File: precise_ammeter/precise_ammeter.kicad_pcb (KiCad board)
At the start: 2 copper layers, 94.9 x 63.9 mm, 105 parts, among them J1 Conn_01x01_Socket, J2 Conn_01x01_Socket, J3 USB4110GFA, J4 Conn_ARM_JTAG_SWD_10, U1 INA121U, U11 STM32G431C6Tx, U12 USBLC6-2P6, U2 TLV9301xDBV, U3 TLV9301xDBV, U4 INA137UA, U5 OPA376xxD, U6 OPA376xxD, U7 TPS7A2433DBVR, U9 LMC7660, Y1 Crystal

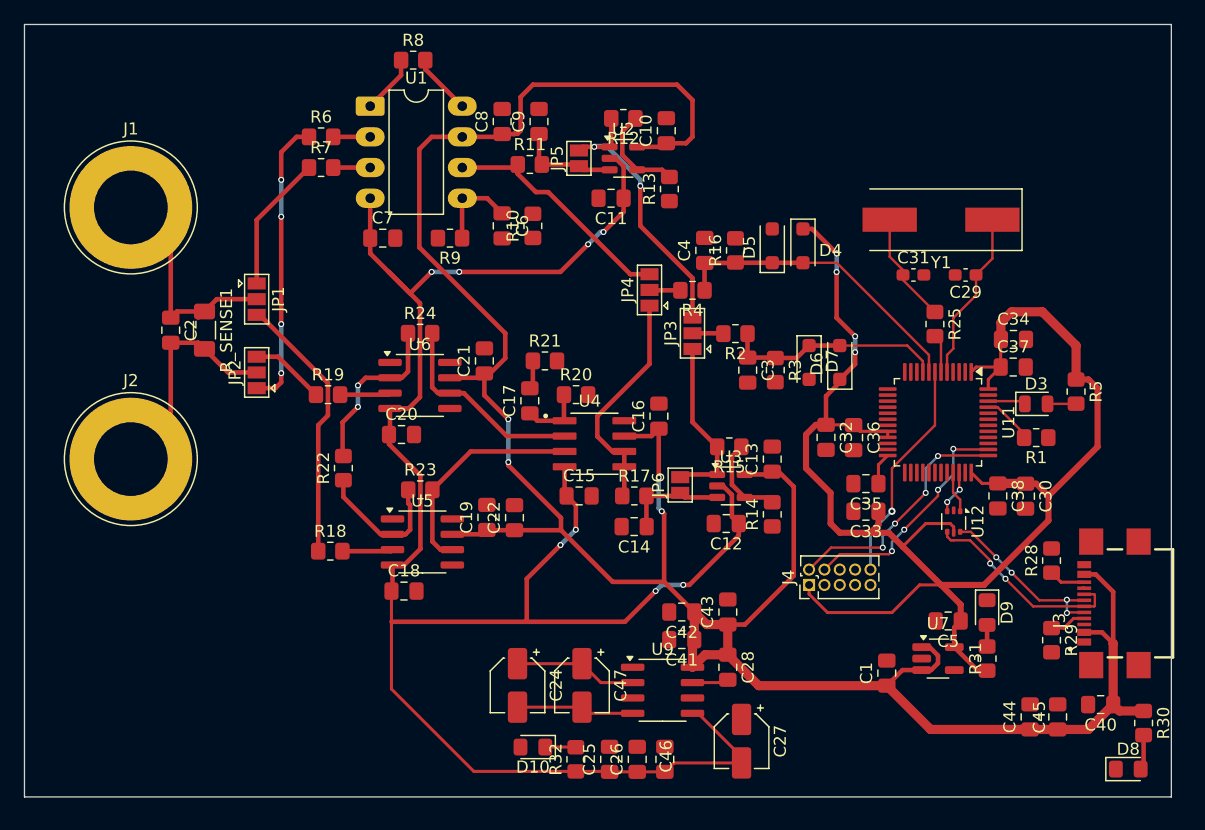
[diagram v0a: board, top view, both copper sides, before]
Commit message: dodano skonczone PCB
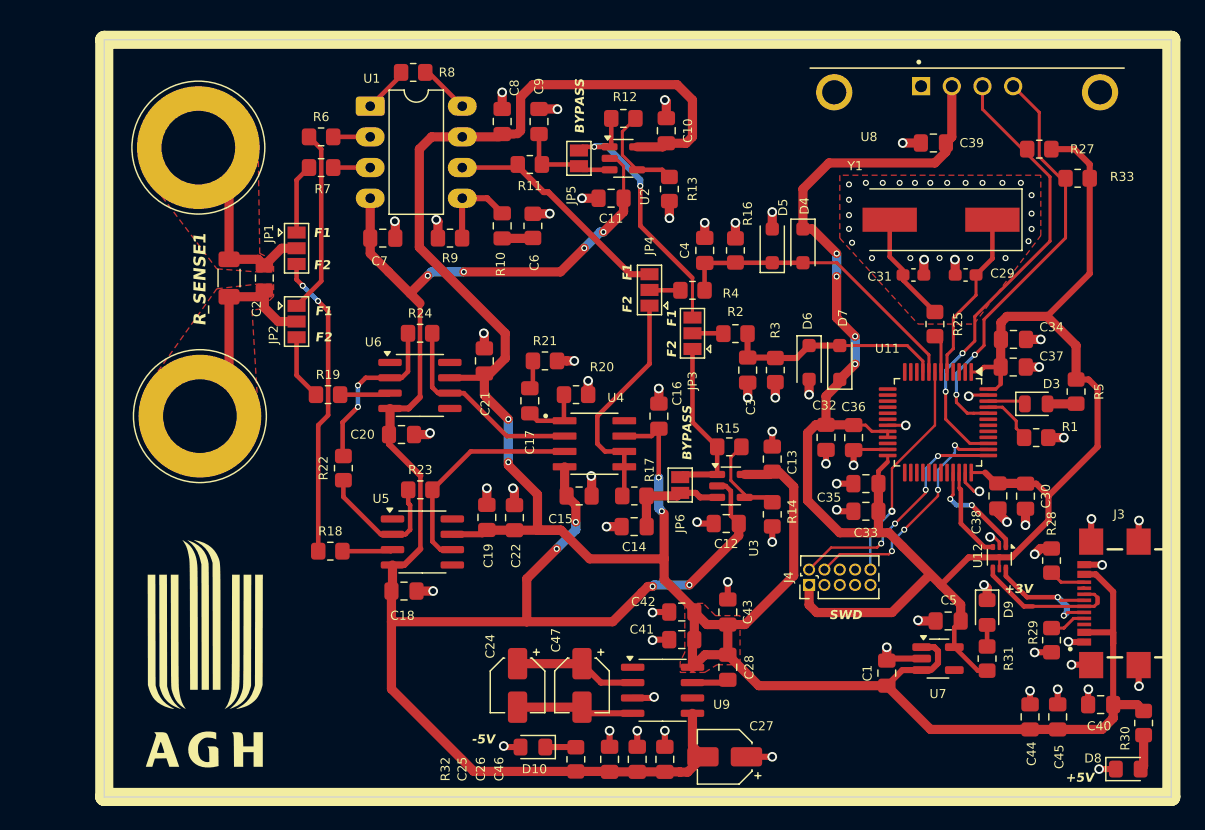
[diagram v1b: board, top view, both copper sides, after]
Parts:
- added C39: 1u, Capacitor_SMD:C_0805_2012Metric_Pad1.18x1.45mm_HandSolder, F.Cu at (213.7, 91.2)
- added G***: LOGO, LOGO, F.Cu at (153.4, 133.5)
- added R27: 4.7k, Resistor_SMD:R_0805_2012Metric_Pad1.20x1.40mm_HandSolder, F.Cu at (222.5, 91.7)
- added R33: 4.7k, Resistor_SMD:R_0805_2012Metric_Pad1.20x1.40mm_HandSolder, F.Cu at (225.7, 94.1)
- added U8: DM-OLED096-636, DM-OLED096-636:MODULE_DM-OLED096-636, F.Cu at (216.5, 98.0)
- moved C2 8.87 mm to (158.4, 102.4)
- moved J1 7.47 mm to (152.9, 91.6)
- moved J2 6.73 mm to (153.0, 113.8)
- moved JP1 5.35 mm to (161.0, 99.9)
- moved JP2 5.35 mm to (161.0, 106.0), turned to -90 degrees
- moved U12 4.80 mm to (219.2, 125.5)
- moved R_SENSE1 4.77 mm to (155.4, 102.4)
- moved C27 1.90 mm to (196.5, 142.0), turned to 180 degrees
- moved R8 1.02 mm to (170.7, 85.3)
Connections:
- U11 pad 39: unconnected-(U11-PA15-Pad39) -> /MCU/SCL
- U11 pad 44: unconnected-(U11-PB7-Pad44) -> /MCU/SDA
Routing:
- net GND: track 0.00 -> 101.1 mm, vias 0 -> 91
- net /MCU/SCL: track 0.00 -> 38.0 mm, vias 0 -> 2
- net +3V3: track 132.2 -> 170.0 mm
- net /MCU/SDA: track 0.00 -> 34.9 mm, vias 0 -> 2
- net /Curr_measurement/Frontend_1/Frontend_1_IN-: track 24.1 -> 15.2 mm, vias 4 -> 0
- net /Curr_measurement/Frontend_1/Frontend_1_IN+: track 11.4 -> 5.81 mm
- net Net-(U11-PA11): track 3.45 -> 9.00 mm, vias 0 -> 2
- net /MCU/USB_D_P: track 17.0 -> 12.2 mm, vias 2 -> 0
- net -5VA: track 165.0 -> 160.6 mm
- net Net-(U11-PA12): track 3.66 -> 7.73 mm, vias 2 -> 0
- net /Curr_measurement/IN-: track 19.1 -> 22.7 mm
- net /MCU/USB_D_N: track 15.2 -> 11.8 mm, vias 4 -> 2
- net /Curr_measurement/Frontend_2/Frontend_2_IN+: track 22.5 -> 25.2 mm, vias 0 -> 2
- net Net-(C6-Pad2): track 0.00 -> 2.56 mm
- net /Curr_measurement/IN+: track 19.0 -> 16.7 mm
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- added copper zone on F.Cu, net +5VA
- added copper zone on F.Cu, net /Curr_measurement/IN+
- added copper zone on F.Cu, net /Curr_measurement/IN-
- added copper zone on B.Cu, net GND
- added copper zone on F.Cu, net GND
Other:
- board size 94.9 x 63.9 mm -> 88.3 x 62.7 mm
- board text added: "+3V"
- board text added: "+5V"
- board text added: "-5V"
- board text added: "Autorzy: - Filip Kulka - Dominik Michalczyk - Krzysztof Sikora Kraków 2025"
- board text added: "BYPASS"
- board text added: "F1"
- board text added: "F2"
- board text added: "SWD"
